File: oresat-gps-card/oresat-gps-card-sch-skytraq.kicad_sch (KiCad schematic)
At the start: 11 parts, among them U23 ORION-B16

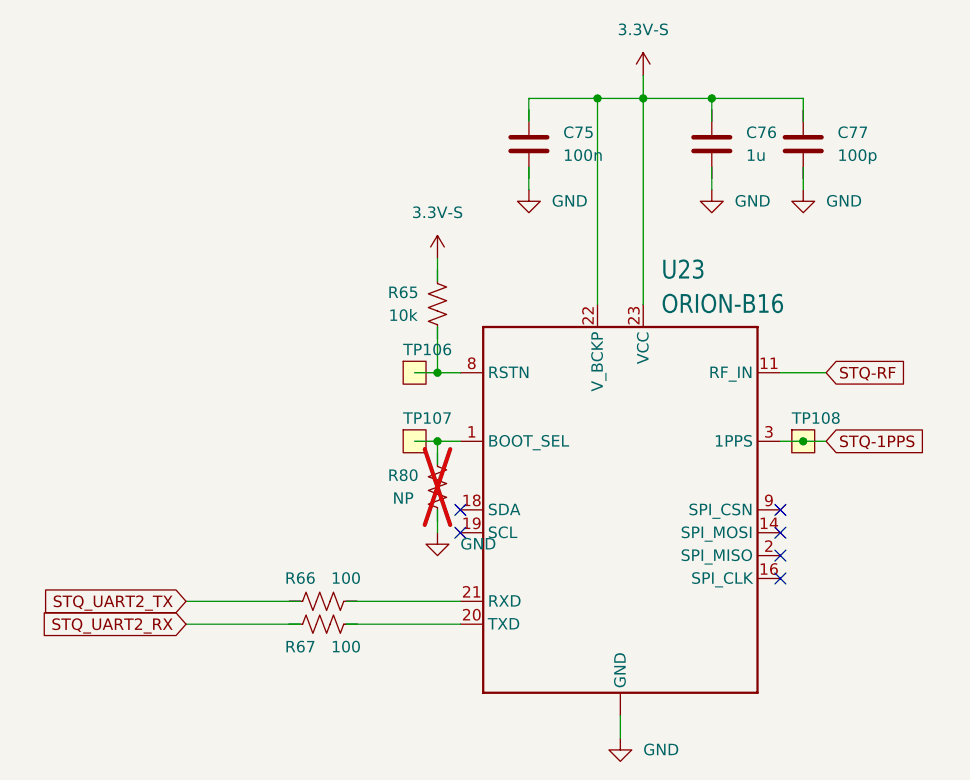
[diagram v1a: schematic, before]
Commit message: Routine Push
Various small changes made
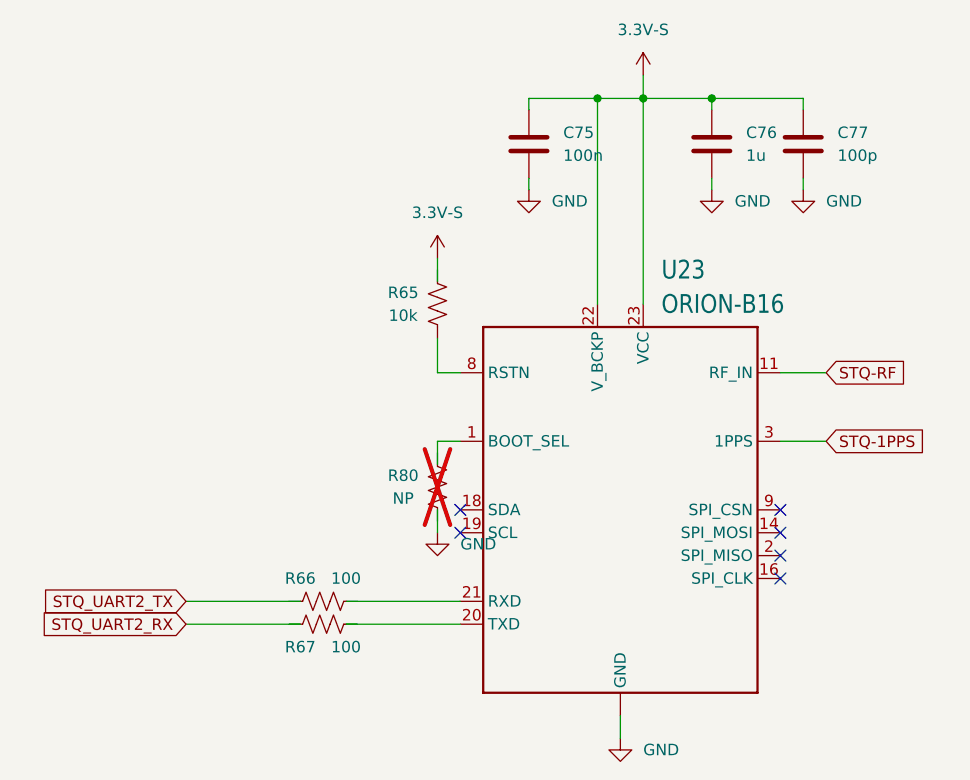
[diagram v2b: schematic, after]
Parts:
- removed TP106, TP107, TP108: 1x01, oresat-misc:TestPoint-0.75mm-th, symbol oresat-misc:Test-Point-0.75mm-th
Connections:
- net 3.3V-S: now also C75.1, C76.1, C77.1
- net GND: now also C75.2, C76.2, C77.2
- net at U23.8 (RSTN): now also R65.2
